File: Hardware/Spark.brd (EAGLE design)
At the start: 29 parts, among them J1 ARDUINO_R3_SHIELD, Q2 MMBT4403, U1 HX711

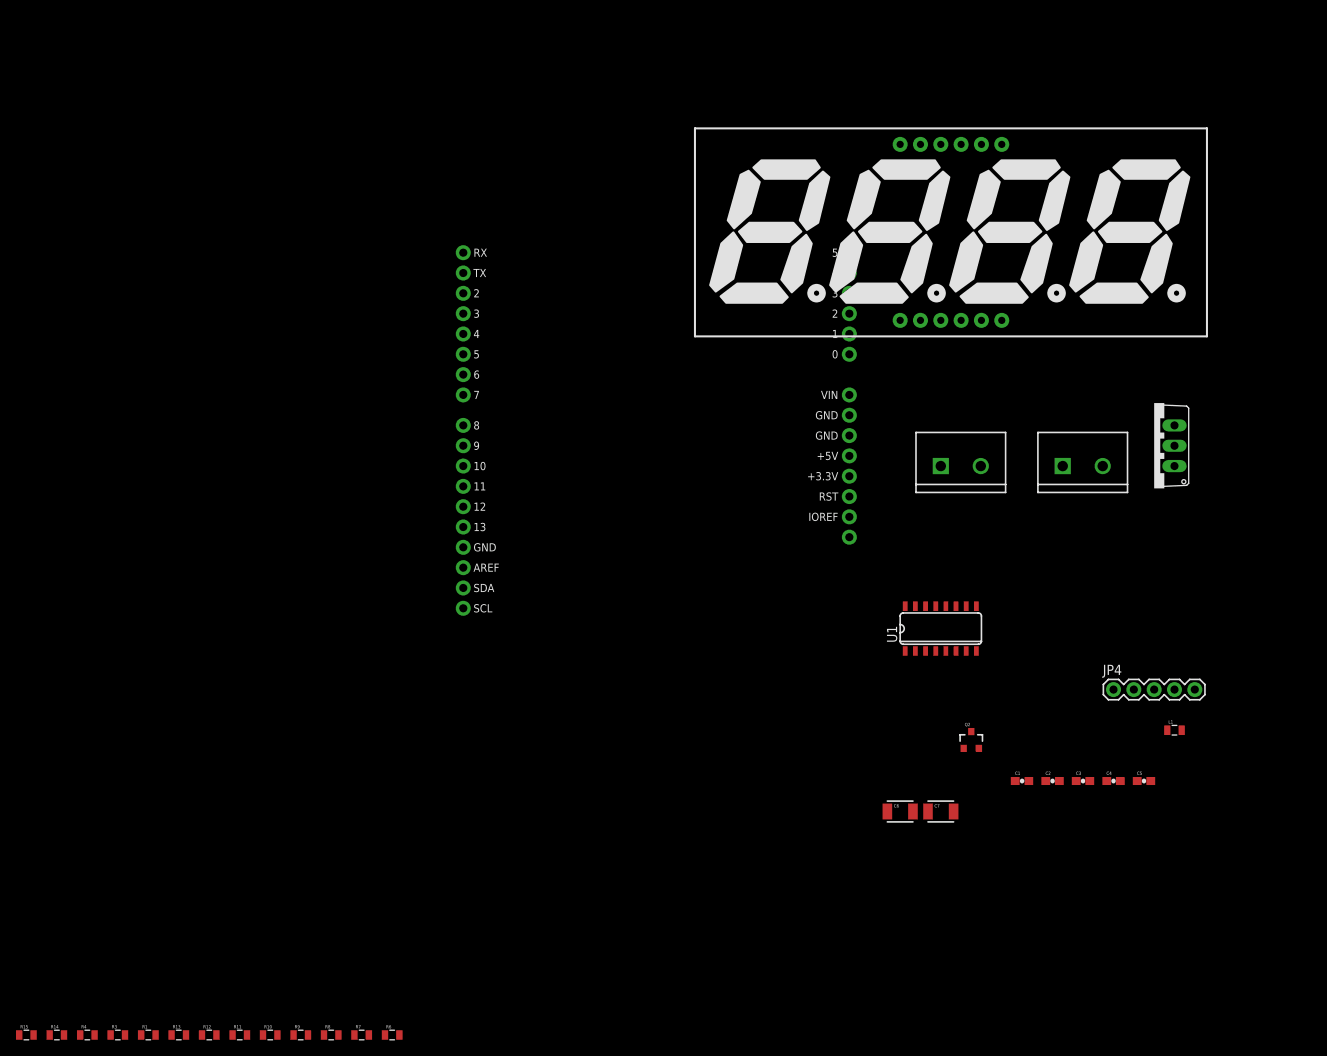
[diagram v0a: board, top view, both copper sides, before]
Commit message: begin layout
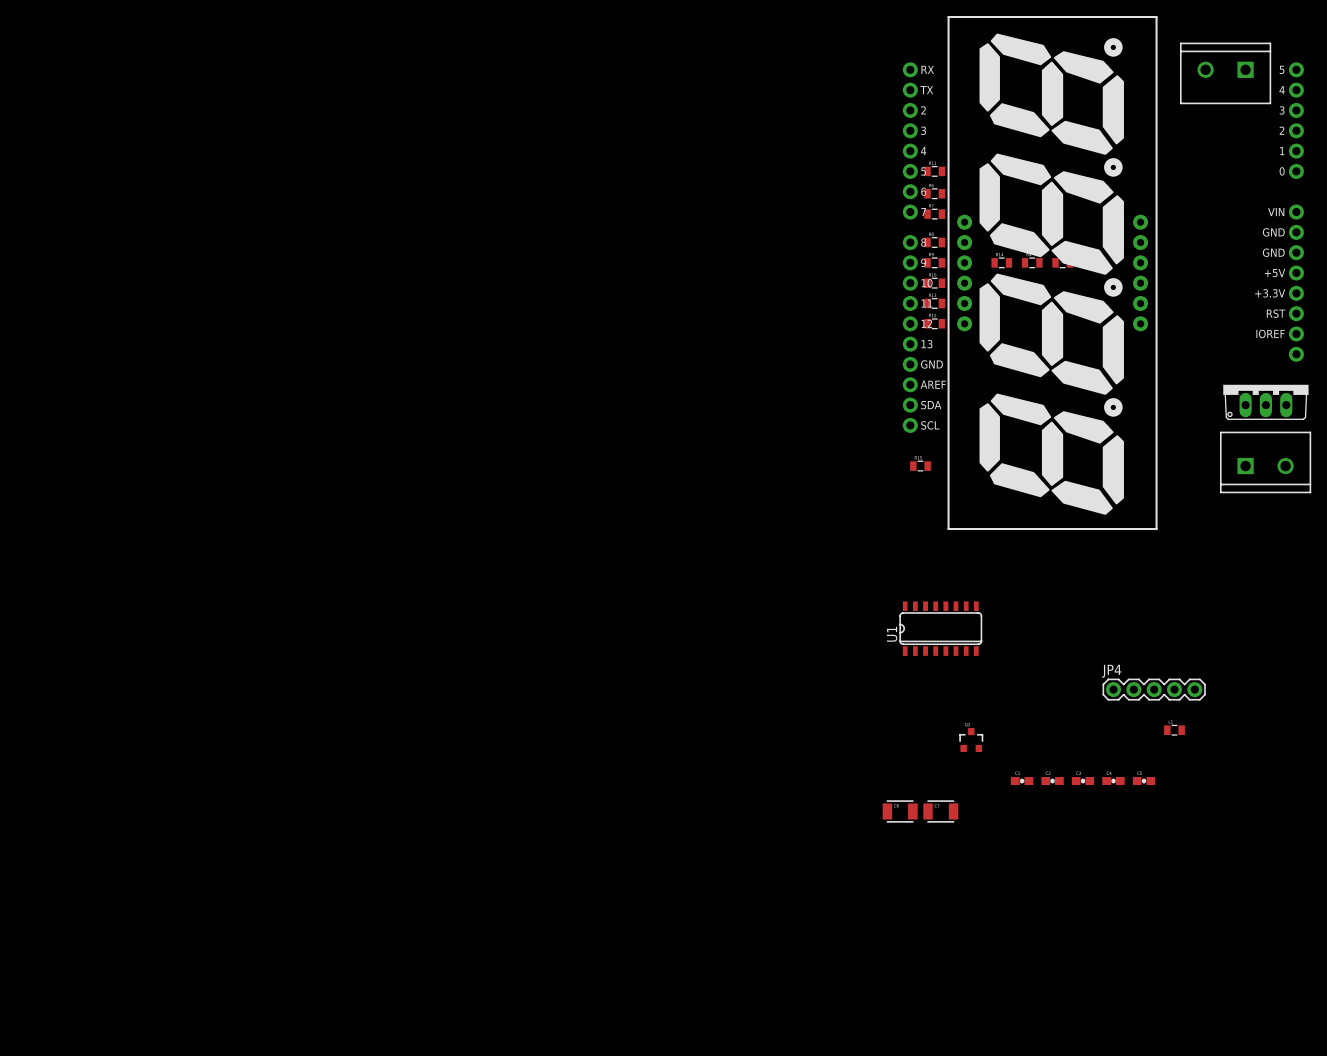
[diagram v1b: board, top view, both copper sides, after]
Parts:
- R1: value (none) -> 10k
- moved R1 152.5 mm to (25.4, 30.5)
- moved R14 152.5 mm to (14.0, 30.5)
- moved R3 152.5 mm to (21.6, 30.5)
- moved R4 152.5 mm to (17.8, 30.5)
- moved R11 138.6 mm to (5.59, 41.9)
- moved R15 132.5 mm to (3.81, 5.08)
- moved R13 131.5 mm to (5.59, 25.4)
- moved R12 127.0 mm to (5.59, 22.9)
- moved R10 125.4 mm to (5.59, 27.9)
- moved R7 125.1 mm to (5.59, 36.6)
- moved R6 125.1 mm to (5.59, 39.1)
- moved R9 124.9 mm to (5.59, 30.5)
- moved R8 124.5 mm to (5.59, 33.0)
- moved J1 60.4 mm to (0.00, 0.00)
- moved JP1 54.6 mm to (44.5, 54.6), turned to 180 degrees
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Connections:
- net A: now also J1.D11; no longer J1.D5
- net D: now also J1.A1; no longer J1.D8
- net DIG3: now also J1.D8; no longer J1.A1
- net G: now also J1.D5; no longer J1.D11
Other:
- board text removed: "+ -"
- board text removed: "10k"
- board text removed: "IGN"
- board text removed: "POWER"
